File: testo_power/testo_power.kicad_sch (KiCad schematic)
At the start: 8 parts, among them J1 Conn_01x06_Pin, J2 Conn_01x02_Socket, J3 Conn_01x02_Socket, Q1 NDP6020P

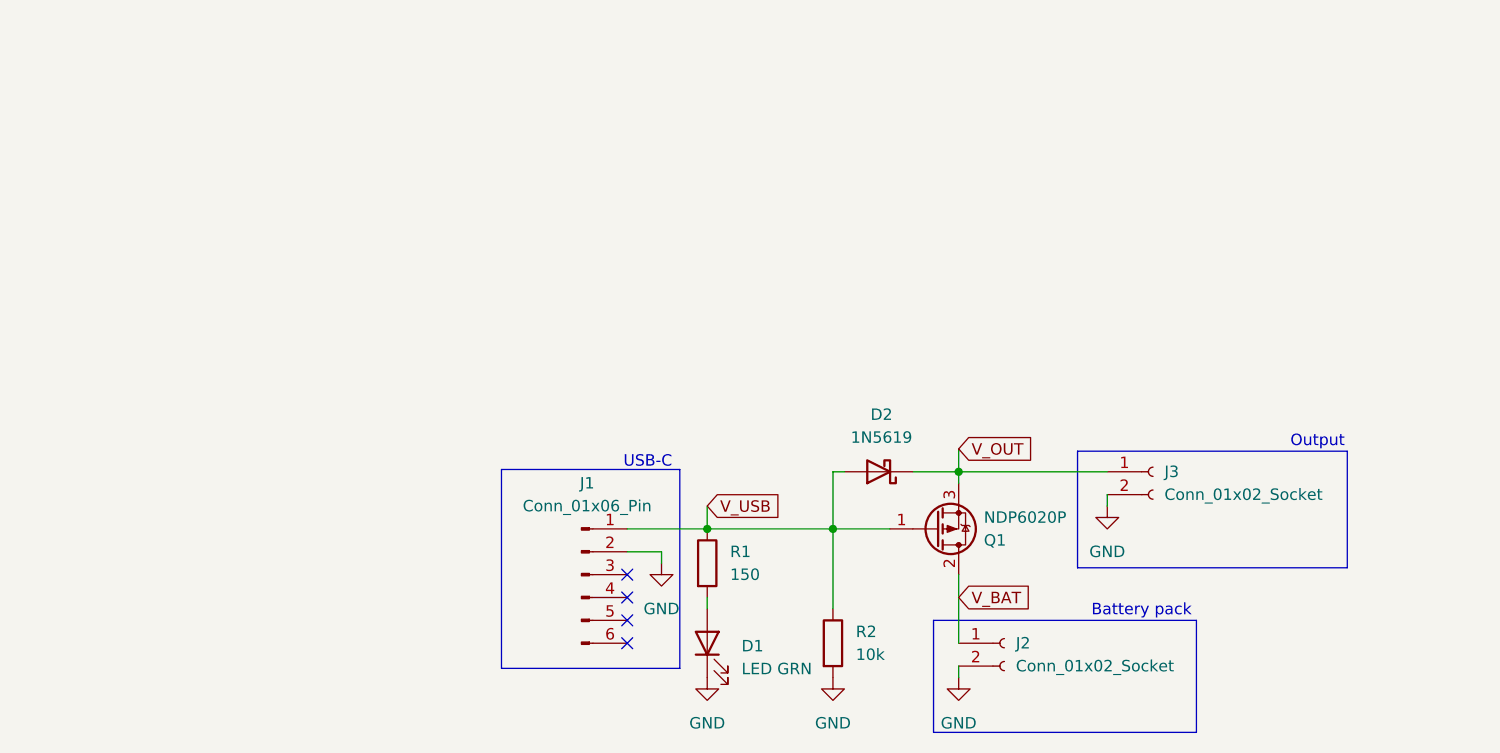
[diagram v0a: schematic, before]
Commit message: pcb and schematic done
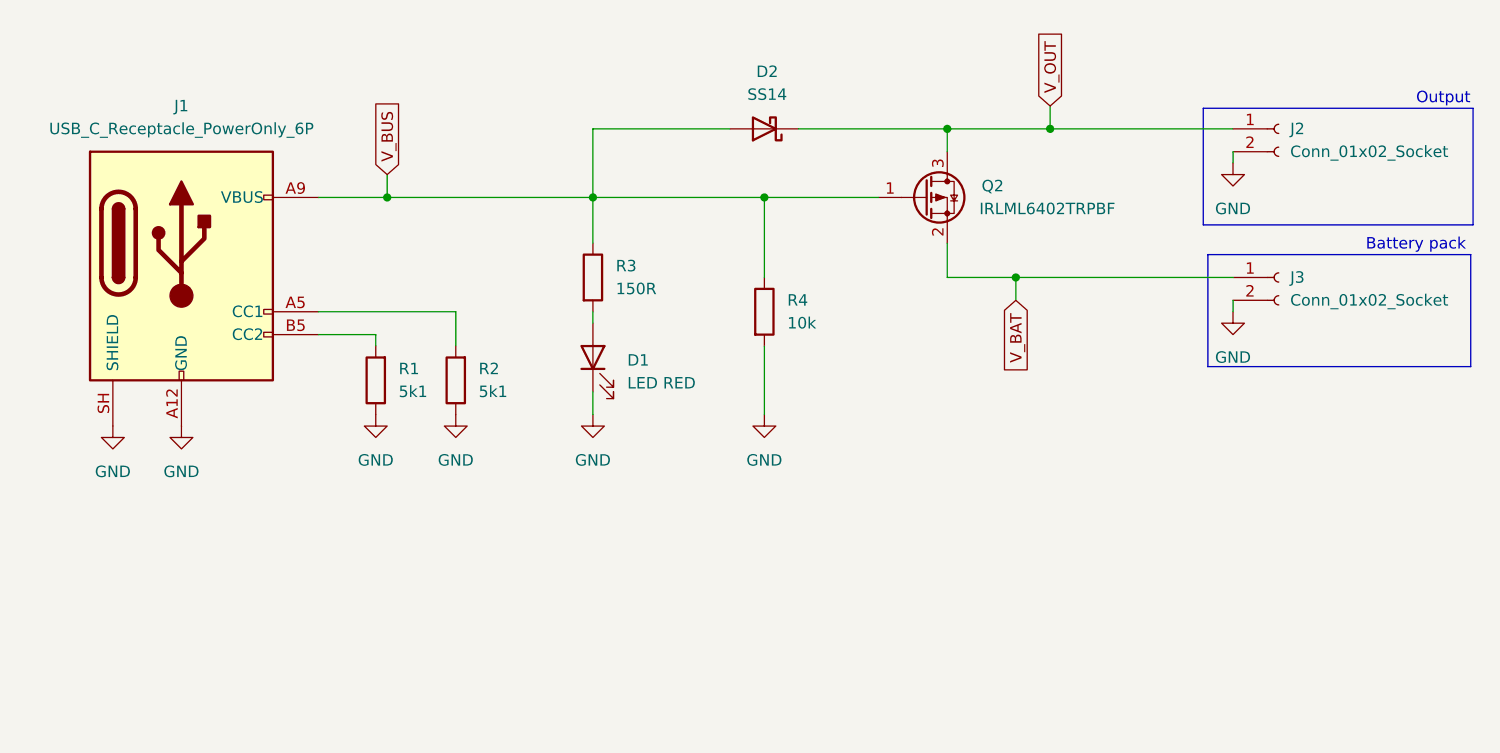
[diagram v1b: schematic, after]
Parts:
- removed J1: Conn_01x06_Pin, Connector_PinHeader_2.54mm:PinHeader_1x06_P2.54mm_Vertical, symbol Connector:Conn_01x06_Pin
- removed Q1: NDP6020P, Package_TO_SOT_THT:TO-220-3_Vertical, symbol Transistor_FET:FQP27P06
- added J1: USB_C_Receptacle_PowerOnly_6P, Connector_USB:USB_C_Receptacle_HCTL_HC-TYPE-C-16P-01A, symbol Connector:USB_C_Receptacle_PowerOnly_6P
- added Q2: IRLML6402TRPBF, Package_TO_SOT_SMD:SOT-23, symbol Transistor_FET:Q_PMOS_GSD
- added R3: 150R, Resistor_SMD:R_0603_1608Metric, symbol Device:R
- added R4: 10k, Resistor_SMD:R_0603_1608Metric, symbol Device:R
- D1: value LED GRN -> LED RED; footprint LED_THT:LED_D4.0mm -> LED_SMD:LED_0603_1608Metric; JLC Part# (none) -> C2286
- D2: value 1N5619 -> SS14; footprint Diode_THT:D_5W_P10.16mm_Horizontal -> Diode_SMD:D_SMA; JLC Part# (none) -> C2480
- J2: footprint Connector_Molex:Molex_KK-254_AE-6410-02A_1x02_P2.54mm_Vertical -> Connector_Molex:Molex_CLIK-Mate_502382-0270_1x02-1MP_P1.25mm_Vertical; JLC Part# (none) -> C27543
- J3: footprint Connector_PinHeader_2.54mm:PinHeader_1x02_P2.54mm_Vertical -> Connector_Molex:Molex_KK-254_AE-6410-02A_1x02_P2.54mm_Vertical; JLC Part# (none) -> C27543
- R1: value 150 -> 5k1; footprint Resistor_THT:R_Axial_DIN0207_L6.3mm_D2.5mm_P7.62mm_Horizontal -> Resistor_SMD:R_0603_1608Metric; JLC Part# (none) -> C23186
- R2: value 10k -> 5k1; footprint Resistor_THT:R_Axial_DIN0207_L6.3mm_D2.5mm_P7.62mm_Horizontal -> Resistor_SMD:R_0603_1608Metric; JLC Part# (none) -> C23186
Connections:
- net GND: now also R1.1, R2.1, J1.A12 (GND), J1.B12 (GND), J1.SH (SHIELD), R4.2; no longer R2.2
- net V_BAT: now also J3.1 (Pin_1), Q2.2 (S); no longer J2.1 (Pin_1)
- net V_OUT: now also J2.1 (Pin_1), Q2.3 (D); no longer J3.1 (Pin_1)
- net at D1.2 (A): now also R3.2; no longer R1.2
- removed net V_USB: D2.2 (A), R1.1, R2.1
- new net: J1.A5 (CC1), R2.2
- new net: J1.B5 (CC2), R1.2
- new net V_BUS: D2.2 (A), J1.A9 (VBUS), J1.B9 (VBUS), Q2.1 (G), R3.1, R4.1
- no-connect marks 4 -> 0
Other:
- note removed: "USB-C"
